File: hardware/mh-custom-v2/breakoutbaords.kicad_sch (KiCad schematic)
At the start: 8 parts, among them J3 Conn_02x19_Top_Bottom, J4 Conn_02x19_Top_Bottom

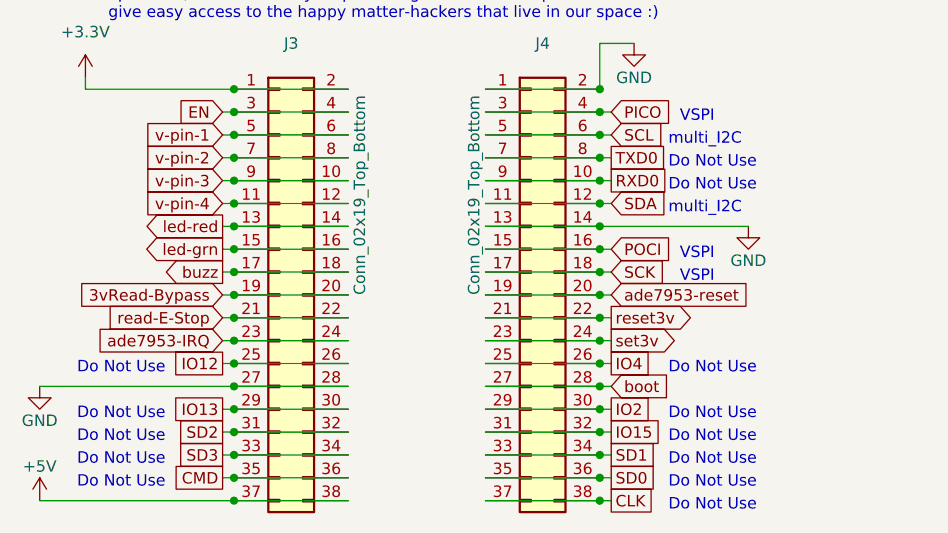
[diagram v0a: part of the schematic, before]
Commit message: approaching ordering from JLCPCB
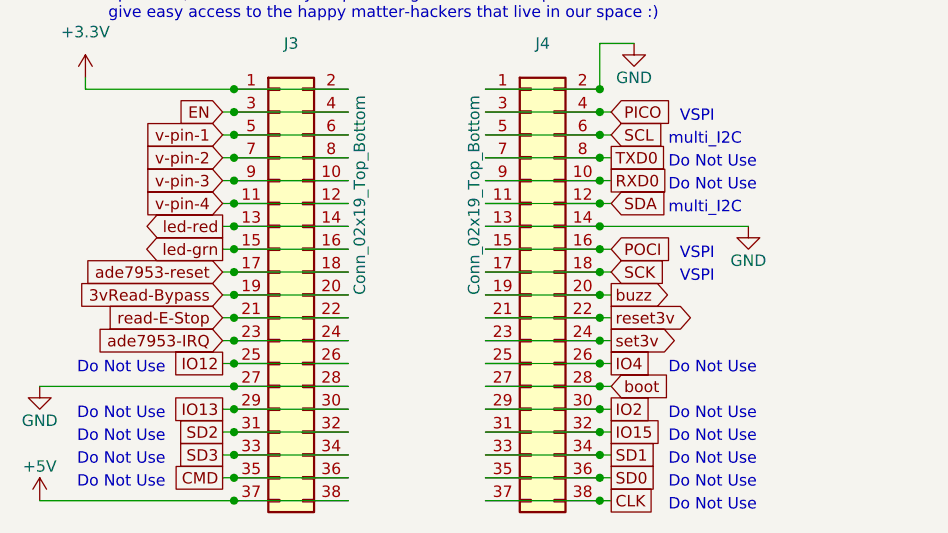
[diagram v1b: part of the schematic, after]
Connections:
- net ade7953-reset: now also J3.17 (Pin_17), J3.18 (Pin_18); no longer J4.19 (Pin_19), J4.20 (Pin_20)
- net buzz: now also J4.19 (Pin_19), J4.20 (Pin_20); no longer J3.17 (Pin_17), J3.18 (Pin_18)
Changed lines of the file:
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@@
   (junction (at 111.76 129.54) (diameter 0) (color 0 0 0 0)
   )
+  (junction (at 111.76 144.78) (diameter 0) (color 0 0 0 0)
+  )
   (junction (at 207.01 92.71) (diameter 0) (color 0 0 0 0)
   )
@@
   (junction (at 111.76 157.48) (diameter 0) (color 0 0 0 0)
   )
+  (junction (at 111.76 142.24) (diameter 0) (color 0 0 0 0)
+  )
+  (junction (at 71.12 162.56) (diameter 0) (color 0 0 0 0)
+  )
+  (junction (at 87.63 35.56) (diameter 0) (color 0 0 0 0)
+  )
+  (junction (at 71.12 132.08) (diameter 0) (color 0 0 0 0)
+  )
   (junction (at 71.12 142.24) (diameter 0) (color 0 0 0 0)
   )
-  (junction (at 111.76 142.24) (diameter 0) (color 0 0 0 0)
-  )
-  (junction (at 71.12 162.56) (diameter 0) (color 0 0 0 0)
-  )
-  (junction (at 87.63 35.56) (diameter 0) (color 0 0 0 0)
-  )
-  (junction (at 71.12 132.08) (diameter 0) (color 0 0 0 0)
-  )
   (junction (at 111.76 167.64) (diameter 0) (color 0 0 0 0)
   )
@@
   (junction (at 111.76 147.32) (diameter 0) (color 0 0 0 0)
   )
-  (junction (at 111.76 144.78) (diameter 0) (color 0 0 0 0)
-  )
   (junction (at 111.76 132.08) (diameter 0) (color 0 0 0 0)
   )
@@
     (stroke (width 0) (type default) (color 0 0 0 0))
   )
+  (wire (pts (xy 111.76 144.78) (xy 113.03 144.78))
+    (stroke (width 0) (type default) (color 0 0 0 0))
+  )
   (wire (pts (xy 99.06 162.56) (xy 111.76 162.56))
     (stroke (width 0) (type default) (color 0 0 0 0))
@@
     (stroke (width 0) (type default) (color 0 0 0 0))
   )
+  (wire (pts (xy 69.85 142.24) (xy 71.12 142.24))
+    (stroke (width 0) (type default) (color 0 0 0 0))
+  )
   (wire (pts (xy 99.06 144.78) (xy 111.76 144.78))
     (stroke (width 0) (type default) (color 0 0 0 0))
@@
     (stroke (width 0) (type default) (color 0 0 0 0))
   )
-  (wire (pts (xy 111.76 144.78) (xy 113.03 144.78))
-    (stroke (width 0) (type default) (color 0 0 0 0))
-  )
   (wire (pts (xy 217.17 90.17) (xy 217.17 91.44))
     (stroke (width 0) (type default) (color 0 0 0 0))
@@
   )
   (wire (pts (xy 111.76 142.24) (xy 113.03 142.24))
-    (stroke (width 0) (type default) (color 0 0 0 0))
-  )
-  (wire (pts (xy 69.85 142.24) (xy 71.12 142.24))
     (stroke (width 0) (type default) (color 0 0 0 0))
   )
@@
     )
   )
-  (global_label "buzz" (shape output) (at 69.85 142.24 180) (fields_autoplaced)
-    (effects (font (size 1.27 1.27)) (justify right))
-    (property "Intersheet References" "${INTERSHEET_REFS}" (id 0) (at 63.0826 142.3194 0)
-      (effects (font (size 1.27 1.27)) (justify right) hide)
+  (global_label "buzz" (shape output) (at 113.03 144.78 0) (fields_autoplaced)
+    (effects (font (size 1.27 1.27)) (justify left))
+    (property "Intersheet References" "${INTERSHEET_REFS}" (id 0) (at 119.7974 144.7006 0)
+      (effects (font (size 1.27 1.27)) (justify left) hide)
     )
   )
@@
     )
   )
-  (global_label "ade7953-reset" (shape input) (at 113.03 144.78 0) (fields_autoplaced)
-    (effects (font (size 1.27 1.27)) (justify left))
-    (property "Intersheet References" "${INTERSHEET_REFS}" (id 0) (at 129.9574 144.8594 0)
-      (effects (font (size 1.27 1.27)) (justify left) hide)
-    )
-  )
+  (global_label "ade7953-reset" (shape input) (at 69.85 142.24 180) (fields_autoplaced)
+    (effects (font (size 1.27 1.27)) (justify right))
+    (property "Intersheet References" "${INTERSHEET_REFS}" (id 0) (at 52.9226 142.1606 0)
+      (effects (font (size 1.27 1.27)) (justify right) hide)
+    )
+  )
